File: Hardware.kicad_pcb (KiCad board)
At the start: 2 copper layers, 80 x 40 mm, 124 parts, among them J1 Conn_01x06_Socket, J2 JAE_SIM_Card_SF72S006, J3 Conn_Coaxial, J4 Conn_Coaxial, J5 Conn_01x05_Socket, J9 Battery, Q1 BC849, Q2 BC849, Q3 MMBT3904, Q4 BC849, Q5 MMBT3904, Q6 MMBT3904, SW1 SW_Push, SW3 SW_Push, U1 ESP32-WROOM-32, U10 MIC29302AWD, U11 AMS1117-3.3, U2 NEO-M8M, U3 SN65HVD231, U4 BQ24075RGT, U5 AT24CS01-XHM, U6 A7670E, U7 AMS1117-3.3, U8 MP1584EN

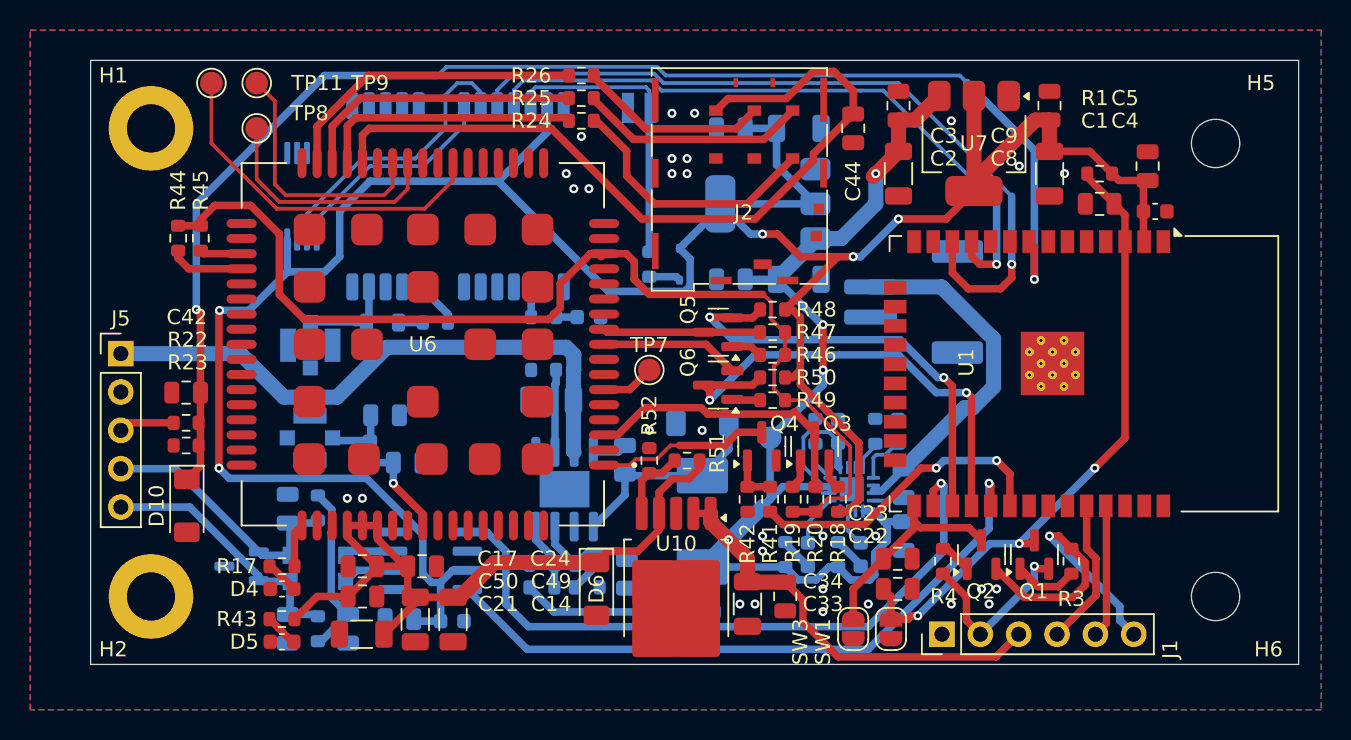
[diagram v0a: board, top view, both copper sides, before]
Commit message: cleaned up
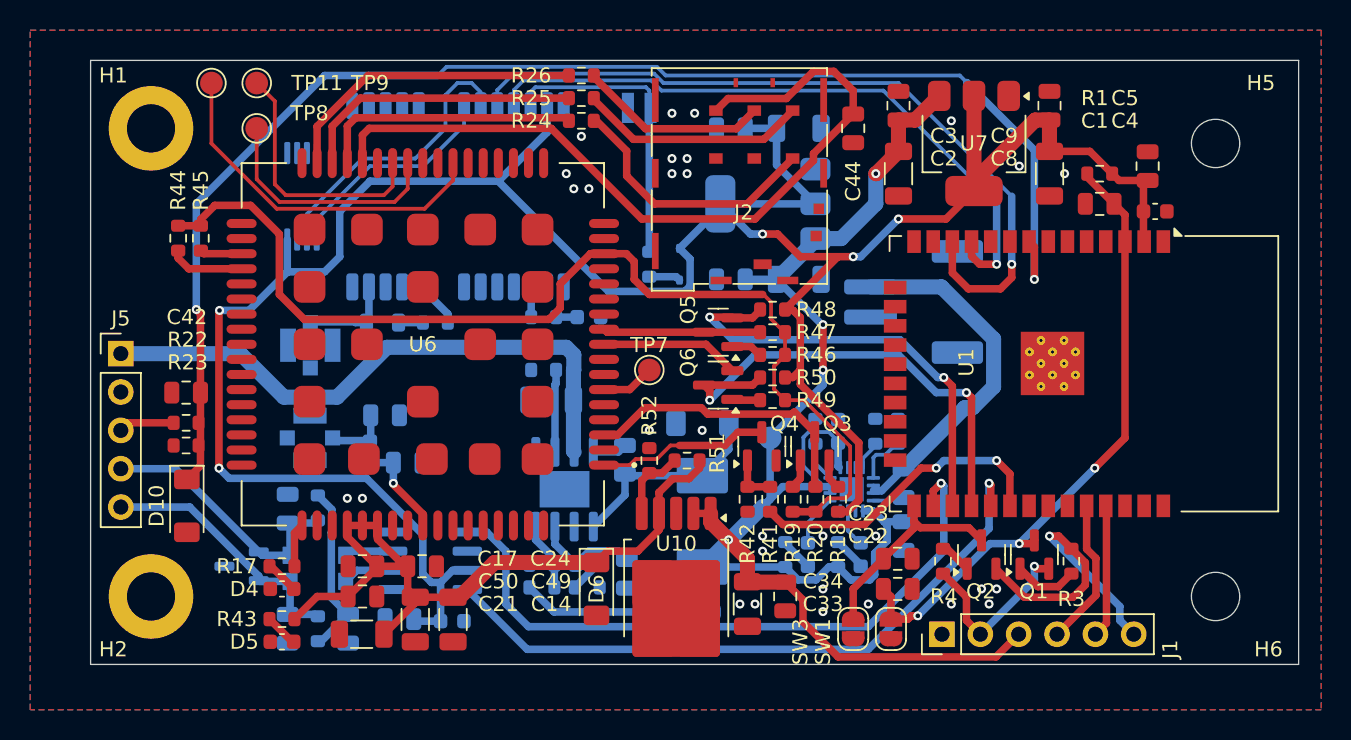
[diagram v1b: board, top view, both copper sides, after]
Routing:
- net +5V: track 121.6 -> 120.2 mm
